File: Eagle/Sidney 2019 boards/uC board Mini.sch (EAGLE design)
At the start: 55 parts

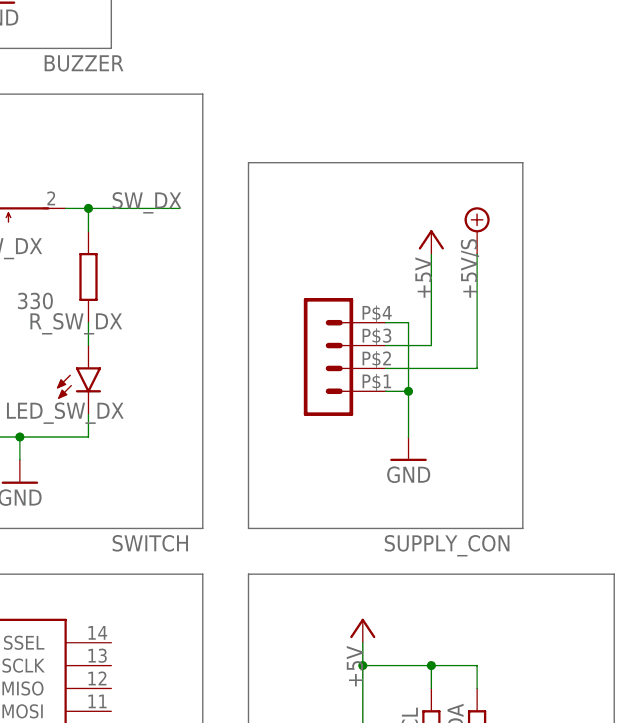
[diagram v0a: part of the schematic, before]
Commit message: general improvements to the boards
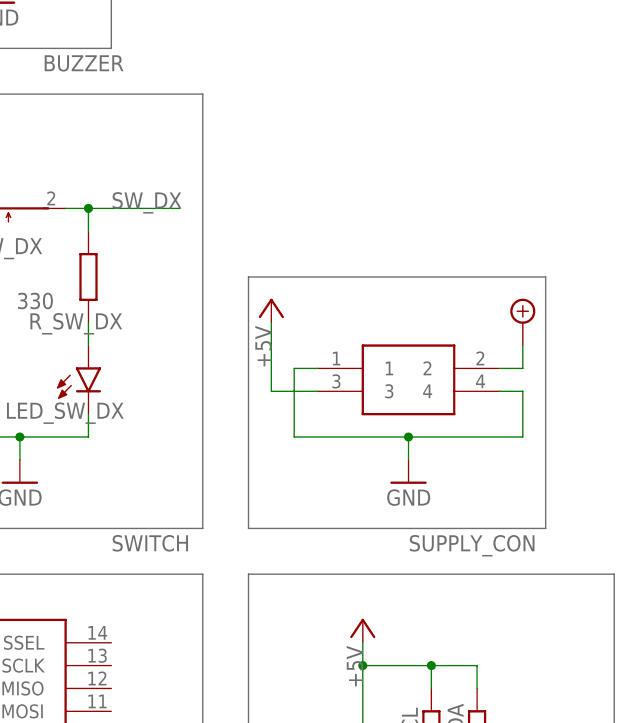
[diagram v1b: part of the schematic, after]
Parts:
- removed SUPPLY_CON: (no value), con-molex-micro-fit-3_0:HEADER_POS4_43045-0412
- added J1: 39-28-1043, 39-28-1043:39-28-1043
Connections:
- net +5V: now also J1.3; no longer SUPPLY_CON.3
- net +5V/S: now also J1.2; no longer SUPPLY_CON.2
- net GND: now also J1.1, J1.4; no longer SUPPLY_CON.1, SUPPLY_CON.4
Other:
- note added: "SUPPLY_CON"
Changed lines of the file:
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@@
 <setting verticaltext="up"/>
 </settings>
-<grid distance="0.1" unitdist="inch" unit="inch" style="lines" multiple="1" display="no" altdistance="0.01" altunitdist="inch" altunit="inch"/>
+<grid distance="0.1" unitdist="inch" unit="inch" style="lines" multiple="1" display="yes" altdistance="0.01" altunitdist="inch" altunit="inch"/>
 <layers>
 <layer number="1" name="Top" color="4" fill="1" visible="no" active="no"/>
@@
 <part name="SUPPLY2" library="supply2" library_urn="urn:adsk.eagle:library:372" deviceset="+5V/1" device=""/>
 <part name="SUPPLY1" library="supply2" library_urn="urn:adsk.eagle:library:372" deviceset="+5V/1" device=""/>
-<part name="SUPPLY_CON" library="con-molex-micro-fit-3_0" deviceset="HEADER_POS4_?" device="43045-0412"/>
-<part name="P+10" library="supply1" library_urn="urn:adsk.eagle:library:371" deviceset="+5V" device=""/>
-<part name="SUPPLY3" library="supply2" library_urn="urn:adsk.eagle:library:372" deviceset="+5V/1" device=""/>
-<part name="GND18" library="supply1" deviceset="GND" device=""/>
 <part name="R_BALL" library="rcl" library_urn="urn:adsk.eagle:library:334" deviceset="R-EU_" device="R1206" package3d_urn="urn:adsk.eagle:package:23540/2" value="330"/>
 <part name="P+1" library="supply1" library_urn="urn:adsk.eagle:library:371" deviceset="+5V" device=""/>
@@
 <part name="P+11" library="supply1" library_urn="urn:adsk.eagle:library:371" deviceset="+5V" device=""/>
 <part name="P+12" library="supply1" library_urn="urn:adsk.eagle:library:371" deviceset="+5V" device=""/>
+<part name="J1" library="39-28-1043" deviceset="39-28-1043" device=""/>
+<part name="GND34" library="supply1" deviceset="GND" device=""/>
+<part name="P+16" library="supply1" library_urn="urn:adsk.eagle:library:371" deviceset="+5V" device=""/>
+<part name="SUPPLY4" library="supply2" library_urn="urn:adsk.eagle:library:372" deviceset="+5V/1" device=""/>
 </parts>
 <sheets>
@@
 <wire x1="391.16" y1="45.72" x2="431.8" y2="45.72" width="0.1524" layer="95"/>
 <wire x1="386.08" y1="99.06" x2="386.08" y2="50.8" width="0.1524" layer="95"/>
-<wire x1="391.16" y1="50.8" x2="391.16" y2="91.44" width="0.1524" layer="95"/>
-<wire x1="391.16" y1="91.44" x2="421.64" y2="91.44" width="0.1524" layer="95"/>
-<wire x1="421.64" y1="91.44" x2="421.64" y2="50.8" width="0.1524" layer="95"/>
-<wire x1="421.64" y1="50.8" x2="391.16" y2="50.8" width="0.1524" layer="95"/>
+<wire x1="391.16" y1="50.8" x2="391.16" y2="78.74" width="0.1524" layer="95"/>
+<wire x1="424.18" y1="50.8" x2="391.16" y2="50.8" width="0.1524" layer="95"/>
 <wire x1="431.8" y1="45.72" x2="431.8" y2="2.54" width="0.1524" layer="95"/>
+<wire x1="424.18" y1="50.8" x2="424.18" y2="78.74" width="0.1524" layer="95"/>
+<wire x1="391.16" y1="78.74" x2="424.18" y2="78.74" width="0.1524" layer="95"/>
+<text x="408.94" y="48.26" size="1.778" layer="95">SUPPLY_CON</text>
 </plain>
 <instances>
@@
 <attribute name="VALUE" x="357.505" y="90.805" size="1.778" layer="96" rot="R90"/>
 </instance>
-<instance part="SUPPLY_CON" gate="G$1" x="401.32" y="71.12" smashed="yes" rot="R180">
-<attribute name="VALUE" x="402.59" y="78.74" size="1.778" layer="96" rot="R180"/>
-<attribute name="NAME" x="420.37" y="50.038" size="1.778" layer="95" rot="R180"/>
-</instance>
-<instance part="P+10" gate="1" x="411.48" y="83.82" smashed="yes">
-<attribute name="VALUE" x="411.48" y="76.2" size="1.778" layer="96" rot="R90"/>
-</instance>
-<instance part="SUPPLY3" gate="G$1" x="416.56" y="83.82" smashed="yes"/>
-<instance part="GND18" gate="1" x="408.94" y="58.42" smashed="yes" rot="MR0">
-<attribute name="VALUE" x="411.48" y="55.88" size="1.778" layer="96" rot="MR0"/>
-</instance>
 <instance part="R_BALL" gate="G$1" x="116.84" y="25.4" smashed="yes">
 <attribute name="NAME" x="113.03" y="26.8986" size="1.778" layer="95"/>
@@
 <attribute name="VALUE" x="154.94" y="53.34" size="1.778" layer="96" rot="R90"/>
 </instance>
+<instance part="J1" gate="G$1" x="398.78" y="68.58" smashed="yes"/>
+<instance part="GND34" gate="1" x="408.94" y="55.88" smashed="yes" rot="MR0">
+<attribute name="VALUE" x="411.48" y="53.34" size="1.778" layer="96" rot="MR0"/>
+</instance>
+<instance part="P+16" gate="1" x="393.7" y="76.2" smashed="yes">
+<attribute name="VALUE" x="393.7" y="68.58" size="1.778" layer="96" rot="R90"/>
+</instance>
+<instance part="SUPPLY4" gate="G$1" x="421.64" y="73.66" smashed="yes"/>
 </instances>
 <busses>
@@
 </segment>
 <segment>
-<pinref part="SUPPLY_CON" gate="G$1" pin="4"/>
-<pinref part="GND18" gate="1" pin="GND"/>
-<wire x1="406.4" y1="73.66" x2="408.94" y2="73.66" width="0.1524" layer="91"/>
-<wire x1="408.94" y1="73.66" x2="408.94" y2="66.04" width="0.1524" layer="91"/>
-<pinref part="SUPPLY_CON" gate="G$1" pin="1"/>
-<wire x1="408.94" y1="66.04" x2="408.94" y2="60.96" width="0.1524" layer="91"/>
-<wire x1="406.4" y1="66.04" x2="408.94" y2="66.04" width="0.1524" layer="91"/>
-<junction x="408.94" y="66.04"/>
+<pinref part="J1" gate="G$1" pin="1"/>
+<wire x1="398.78" y1="68.58" x2="396.24" y2="68.58" width="0.1524" layer="91"/>
+<wire x1="396.24" y1="68.58" x2="396.24" y2="60.96" width="0.1524" layer="91"/>
+<wire x1="396.24" y1="60.96" x2="408.94" y2="60.96" width="0.1524" layer="91"/>
+<wire x1="408.94" y1="60.96" x2="421.64" y2="60.96" width="0.1524" layer="91"/>
+<wire x1="421.64" y1="60.96" x2="421.64" y2="66.04" width="0.1524" layer="91"/>
+<pinref part="J1" gate="G$1" pin="4"/>
+<wire x1="421.64" y1="66.04" x2="419.1" y2="66.04" width="0.1524" layer="91"/>
+<pinref part="GND34" gate="1" pin="GND"/>
+<wire x1="408.94" y1="58.42" x2="408.94" y2="60.96" width="0.1524" layer="91"/>
+<junction x="408.94" y="60.96"/>
 </segment>
 </net>
@@
 </segment>
 <segment>
-<pinref part="SUPPLY_CON" gate="G$1" pin="3"/>
-<wire x1="406.4" y1="71.12" x2="411.48" y2="71.12" width="0.1524" layer="91"/>
-<pinref part="P+10" gate="1" pin="+5V"/>
-<wire x1="411.48" y1="81.28" x2="411.48" y2="71.12" width="0.1524" layer="91"/>
-</segment>
-<segment>
 <wire x1="330.2" y1="127" x2="330.2" y2="116.84" width="0.1524" layer="91"/>
 <pinref part="BLUETOOTH" gate="1" pin="5"/>
@@
 <wire x1="154.94" y1="50.8" x2="154.94" y2="58.42" width="0.1524" layer="91"/>
 <pinref part="P+12" gate="1" pin="+5V"/>
+</segment>
+<segment>
+<pinref part="J1" gate="G$1" pin="3"/>
+<wire x1="398.78" y1="66.04" x2="393.7" y2="66.04" width="0.1524" layer="91"/>
+<pinref part="P+16" gate="1" pin="+5V"/>
+<wire x1="393.7" y1="73.66" x2="393.7" y2="66.04" width="0.1524" layer="91"/>
 </segment>
 </net>
@@
 </segment>
 <segment>
-<pinref part="SUPPLY_CON" gate="G$1" pin="2"/>
-<wire x1="406.4" y1="68.58" x2="416.56" y2="68.58" width="0.1524" layer="91"/>
-<pinref part="SUPPLY3" gate="G$1" pin="+5V/1"/>
-<wire x1="416.56" y1="68.58" x2="416.56" y2="81.28" width="0.1524" layer="91"/>
-<label x="416.56" y="76.2" size="1.778" layer="95" rot="R90"/>
-</segment>
-<segment>
 <pinref part="P+14" gate="G$1" pin="+5V/1"/>
 <pinref part="R_SDA1" gate="G$1" pin="2"/>
@@
 <wire x1="142.24" y1="90.17" x2="146.05" y2="90.17" width="0.1524" layer="91"/>
 </segment>
-</net>
+<segment>
+<pinref part="J1" gate="G$1" pin="2"/>
+<wire x1="419.1" y1="68.58" x2="421.64" y2="68.58" width="0.1524" layer="91"/>
+<pinref part="SUPPLY4" gate="G$1" pin="+5V/1"/>
+<wire x1="421.64" y1="68.58" x2="421.64" y2="71.12" width="0.1524" layer="91"/>
+</segment>
+</net>
